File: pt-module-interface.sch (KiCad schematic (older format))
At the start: 8 parts

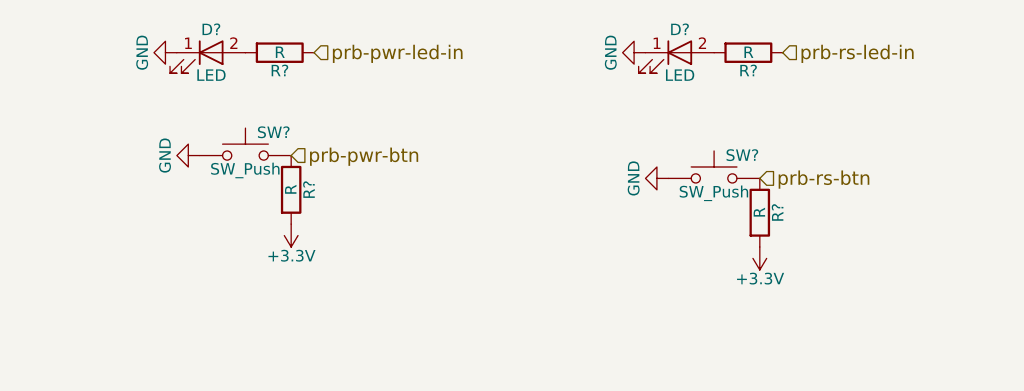
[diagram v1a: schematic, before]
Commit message: add resistor values
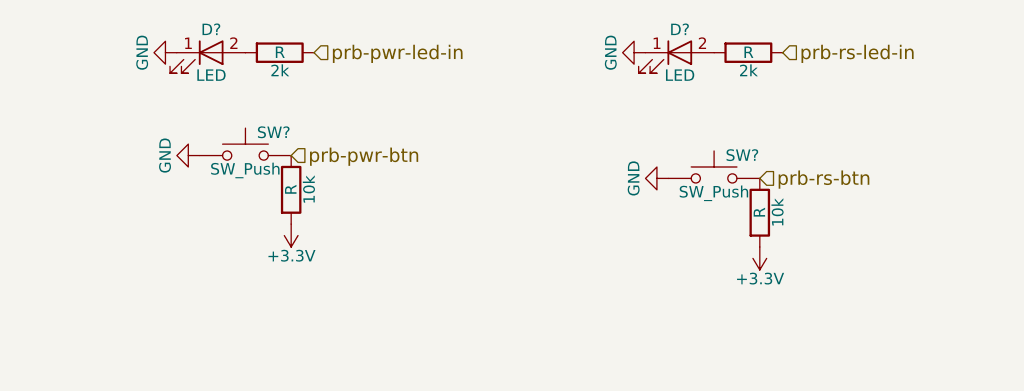
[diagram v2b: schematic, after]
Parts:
- gave numbers to parts that had none: 2
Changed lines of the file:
@@
 $EndComp
 $Comp
-L R R?
+L R 2k
 U 1 1 59819AA1
 P 3250 2450
-F 0 "R?" V 3330 2450 50  0000 C CNN
+F 0 "2k" V 3330 2450 50  0000 C CNN
 F 1 "R" V 3250 2450 50  0000 C CNN
 F 2 "" V 3180 2450 50  0001 C CNN
@@
 $EndComp
 $Comp
-L R R?
+L R 2k
 U 1 1 59819AD9
 P 5300 2450
-F 0 "R?" V 5380 2450 50  0000 C CNN
+F 0 "2k" V 5380 2450 50  0000 C CNN
 F 1 "R" V 5300 2450 50  0000 C CNN
 F 2 "" V 5230 2450 50  0001 C CNN
@@
 $EndComp
 $Comp
-L R R?
+L R 10k
 U 1 1 5981A7B1
 P 3300 3050
-F 0 "R?" V 3380 3050 50  0000 C CNN
+F 0 "10k" V 3380 3050 50  0000 C CNN
 F 1 "R" V 3300 3050 50  0000 C CNN
 F 2 "" V 3230 3050 50  0001 C CNN
@@
 $EndComp
 $Comp
-L R R?
+L R 10k
 U 1 1 5981AB70
 P 5350 3150
-F 0 "R?" V 5430 3150 50  0000 C CNN
+F 0 "10k" V 5430 3150 50  0000 C CNN
 F 1 "R" V 5350 3150 50  0000 C CNN
 F 2 "" V 5280 3150 50  0001 C CNN

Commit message: Added resistor and capacitor values in MCU sheet.
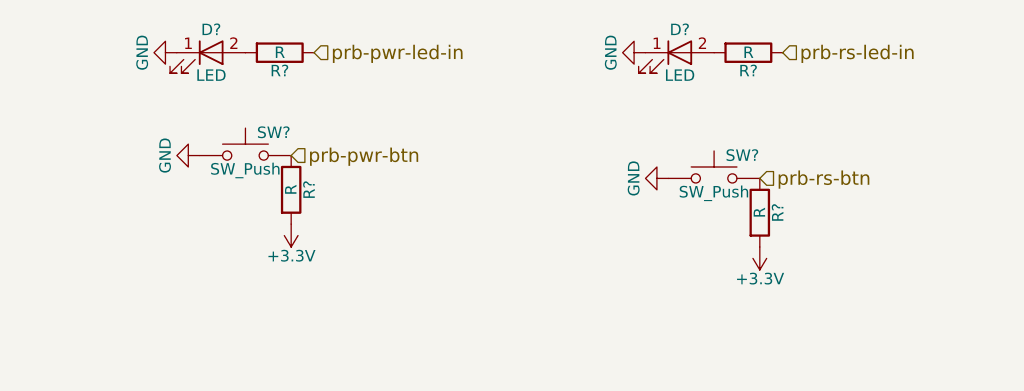
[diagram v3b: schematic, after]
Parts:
- renumbered 2k to R?, 10k to R?
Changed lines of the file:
@@
 $EndComp
 $Comp
-L R 2k
+L R R?
 U 1 1 59819AA1
 P 3250 2450
-F 0 "2k" V 3330 2450 50  0000 C CNN
+F 0 "R?" V 3330 2450 50  0000 C CNN
 F 1 "R" V 3250 2450 50  0000 C CNN
 F 2 "" V 3180 2450 50  0001 C CNN
@@
 $EndComp
 $Comp
-L R 2k
+L R R?
 U 1 1 59819AD9
 P 5300 2450
-F 0 "2k" V 5380 2450 50  0000 C CNN
+F 0 "R?" V 5380 2450 50  0000 C CNN
 F 1 "R" V 5300 2450 50  0000 C CNN
 F 2 "" V 5230 2450 50  0001 C CNN
@@
 $EndComp
 $Comp
-L R 10k
+L R R?
 U 1 1 5981A7B1
 P 3300 3050
-F 0 "10k" V 3380 3050 50  0000 C CNN
+F 0 "R?" V 3380 3050 50  0000 C CNN
 F 1 "R" V 3300 3050 50  0000 C CNN
 F 2 "" V 3230 3050 50  0001 C CNN
@@
 $EndComp
 $Comp
-L R 10k
+L R R?
 U 1 1 5981AB70
 P 5350 3150
-F 0 "10k" V 5430 3150 50  0000 C CNN
+F 0 "R?" V 5430 3150 50  0000 C CNN
 F 1 "R" V 5350 3150 50  0000 C CNN
 F 2 "" V 5280 3150 50  0001 C CNN

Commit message: I don't know what I did
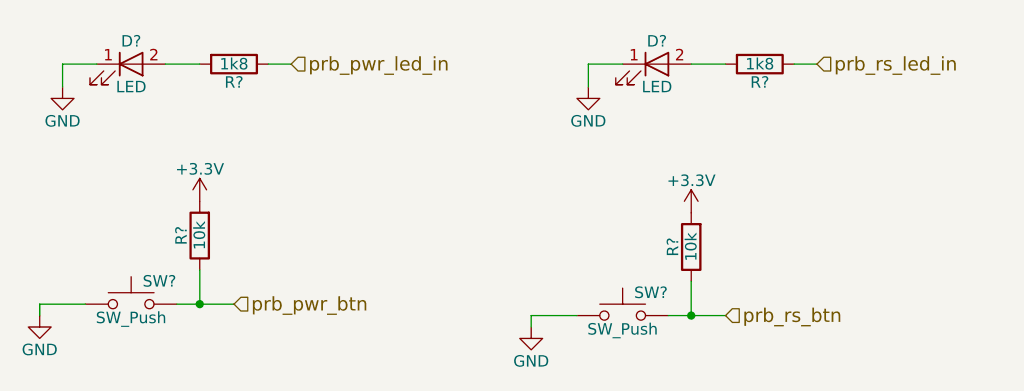
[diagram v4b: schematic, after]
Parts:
- removed D?: LED, symbol LED
- removed R? (x2): R, symbol R
- removed SW?: SW_Push, symbol SW_Push
- added D?: LED, symbol LED
- added R?: 10k, symbol R
- added R?: 1k8, symbol R
- added SW?: SW_Push, symbol SW_Push
- R?: value R -> 1k8
- R?: value R -> 10k
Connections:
- net +3V3: now also R?.2
- net GND: now also D?.1 (K), SW?.1
- net prb-pwr-btn renamed prb_pwr_btn
- net prb-pwr-led-in renamed prb_pwr_led_in
- new net: D?.2 (A), R?.2
- new net prb_rs_btn: R?.1, SW?.2
- new net prb_rs_led_in: R?.1
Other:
- moved on the sheet: D?, R?, SW?
